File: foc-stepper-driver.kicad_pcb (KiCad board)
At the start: 4 copper layers, 42 x 42 mm, 70 parts, among them CN1 XT30UPB-F30.G.Y, J1 Conn_01x04_Pin, J2 TC2030, J3 CAN_CONNECTOR, J4 USART CONNECTOR, U1 DRV8962DDWR, U2 TYPE-C 16PLT-H10.0, U3 STM32G431CBT6, U6 AS5047P-ATSM, U7 TPS560430XDBVR, U8 SPX3819M5-L-3-3/TR, U9 TCAN3403DRQ1, X1 NX3215SA 32.768KHZ EXS00A-MU0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, X2 NDK NX2016SA-24MHZ-EXS00A-CS1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

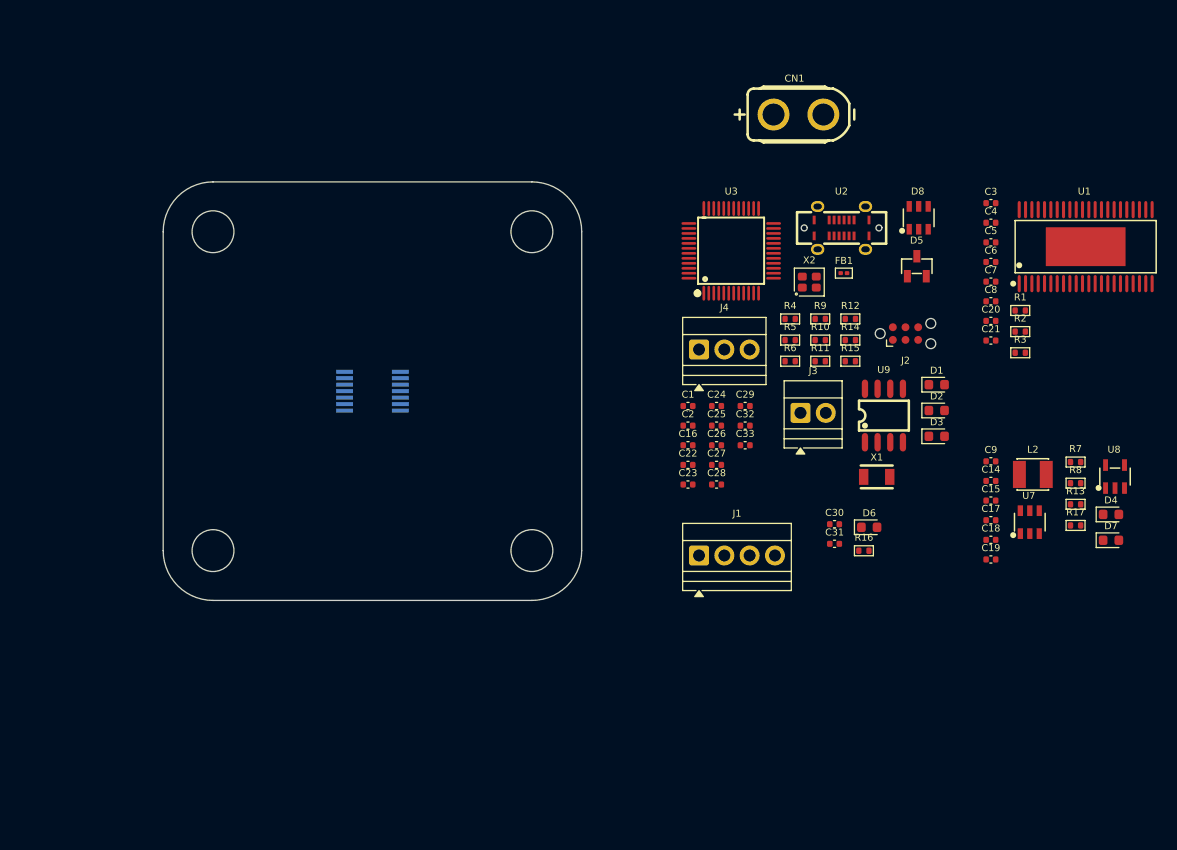
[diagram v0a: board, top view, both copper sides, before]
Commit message: pcb layout
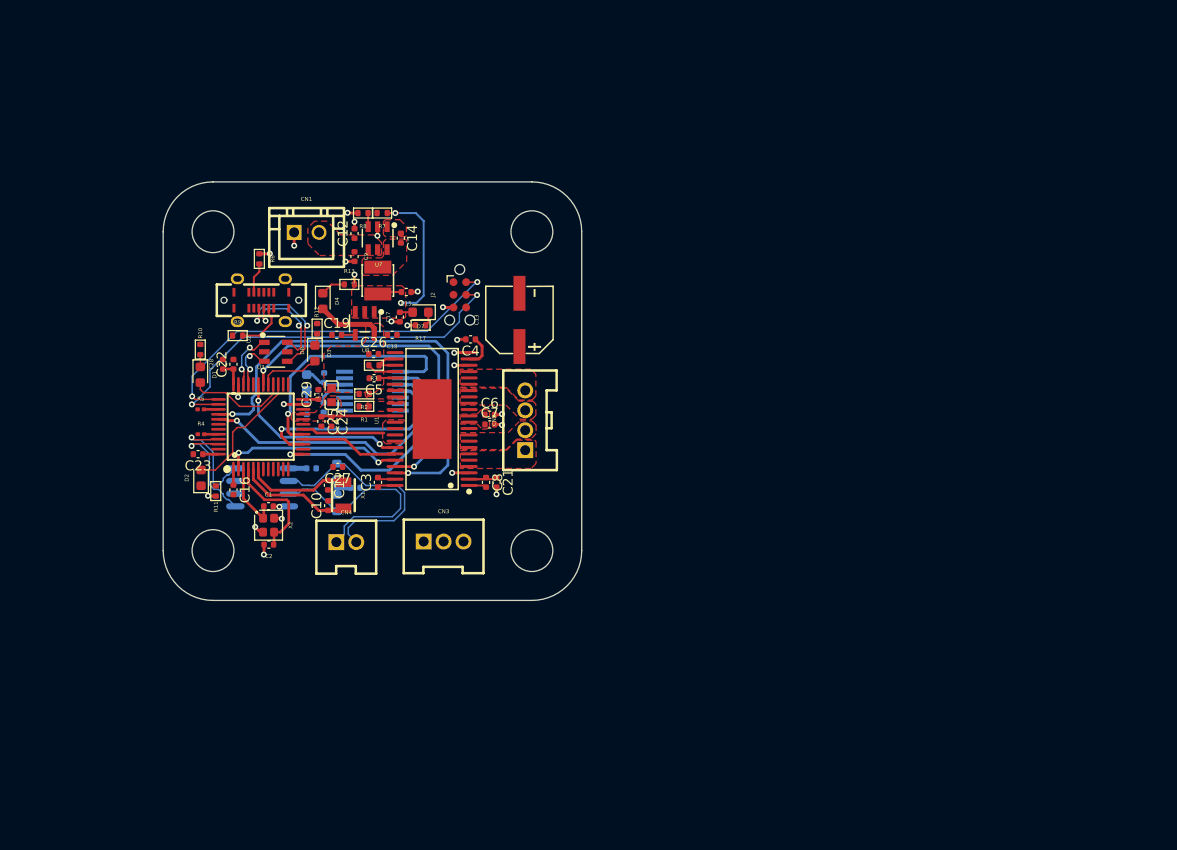
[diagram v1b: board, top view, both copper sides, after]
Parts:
- removed C20: 47u, Capacitor_SMD:C_0402_1005Metric
- removed D5: ESD2CANFD24DBZR, EasyEDA_Lib:SOT-23-3_L2.9-W1.3-P1.90-LS2.4-BL-2
- removed FB1: 120R, PCM_Ferrite_SMD_AKL:Ferrite_0201_0603Metric
- removed J1: Conn_01x04_Pin, TerminalBlock:TerminalBlock_Xinya_XY308-2.54-4P_1x04_P2.54mm_Horizontal
- removed J3: CAN_CONNECTOR, TerminalBlock:TerminalBlock_Xinya_XY308-2.54-2P_1x02_P2.54mm_Horizontal
- removed J4: USART CONNECTOR, TerminalBlock:TerminalBlock_Xinya_XY308-2.54-3P_1x03_P2.54mm_Horizontal
- added C10: 5.1p, Capacitor_SMD:C_0402_1005Metric, F.Cu at (130.9, 96.0)
- added C11: 5.1p, Capacitor_SMD:C_0402_1005Metric, F.Cu at (130.8, 93.9)
- added C12: 100n, Capacitor_SMD:C_0402_1005Metric, F.Cu at (133.5, 68.7)
- added C13: 47uF, EasyEDA_Lib:CAP-SMD_BD6.3-L6.6-W6.6-LS7.3-FD, F.Cu at (150.1, 77.3)
- added CN2: C2839706, EasyEDA_Lib:CONN-TH_PA-4A, F.Cu at (150.6, 87.4)
- added CN3: C2839705, EasyEDA_Lib:CONN-TH_PA-3A, F.Cu at (142.4, 99.6)
- added CN4: C2839704, EasyEDA_Lib:CONN-TH_PA-2A, F.Cu at (132.7, 99.7)
- added L1: BLM18PG121SN1D, EasyEDA_Lib:L0603, F.Cu at (131.2, 84.9)
- C14: value 0.1u -> 100n
- C30, C31, C32, D6, U9: moved to B.Cu
- C33: value 47u -> 4.7n; moved to B.Cu
- C9: value 2.2u -> 10u
- CN1: value XT30UPB-F30.G.Y -> C42391660; footprint EasyEDA_Lib:CONN-TH_XT30UPB-F -> EasyEDA_Lib:CONN-TH_2P-P2.50_HX-2.54MM-2P-ZZ-MS
- R14, R15: footprint PCM_Resistor_SMD_AKL:R_0402_1005Metric -> PCM_Resistor_SMD_AKL:R_0603_1608Metric; moved to B.Cu
- R16: value 100 -> 1k; moved to B.Cu
- R4, R5: footprint PCM_Resistor_SMD_AKL:R_0402_1005Metric -> Capacitor_SMD:C_0201_0603Metric
- moved D4 81.9 mm to (130.3, 75.5), turned to -90 degrees
- moved U8 76.8 mm to (134.5, 77.7), turned to 180 degrees
- moved R8 76.5 mm to (134.3, 66.6), turned to 180 degrees
- moved R13 76.1 mm to (133.0, 73.8)
- moved D2 74.1 mm to (118.1, 93.2), turned to 90 degrees
- moved R7 73.9 mm to (136.3, 66.6), turned to 180 degrees
- moved D1 73.9 mm to (118.0, 82.8), turned to -90 degrees
- moved D7 73.0 mm to (140.1, 76.6), turned to 180 degrees
- moved U7 71.4 mm to (135.8, 69.1), turned to 180 degrees
- moved C19 69.4 mm to (131.7, 78.8)
- moved R17 68.7 mm to (140.1, 77.9), turned to 180 degrees
- moved L2 68.6 mm to (135.8, 73.4), turned to 90 degrees
- moved U1 67.8 mm to (141.3, 87.3), turned to 90 degrees
- moved C3 67.6 mm to (135.8, 93.7), turned to 90 degrees
- moved C9 67.1 mm to (133.5, 71.0), turned to -90 degrees
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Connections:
- net /STM32G431CBT6/STM32_CANFD_RX renamed /STM32G431CBT6/STM32_CANFD+
- net /STM32G431CBT6/STM32_CANFD_TX renamed /STM32G431CBT6/STM32_CANFD-
- net Net-(J3-Pin_1) renamed /STM32G431CBT6/CAN_CONN+
- net Net-(J3-Pin_2) renamed /STM32G431CBT6/CAN_CONN-
- net Net-(U2-DN1) renamed /STM32G431CBT6/USBC_CONN_D-
- net Net-(U2-DP1) renamed /STM32G431CBT6/USBC_CONN_D+
- C19 pad 2: GND -> Net-(U8-BYP)
- C31 pad 2: Net-(D6-K) -> Net-(D6-A)
- C32 pad 1: Net-(U9-VCC) -> +3.3V
- CN1 pad 1: +24V -> GND
- CN1 pad 2: GND -> +24V
- J2 pad 3: /STM32G431CBT6/STM32_NRST -> unconnected-(J2-Pad3)
- R16 pad 1: Net-(D6-A) -> Net-(D6-K)
- U3 pad 14: /DRV8962DDWR/DRV8962_IPROPI1 -> /DRV8962DDWR/DRV8962_IPROPI3
- U3 pad 16: /DRV8962DDWR/DRV8962_IN4 -> /DRV8962DDWR/DRV8962_IN3
- U3 pad 31: /DRV8962DDWR/DRV8962_IN3 -> /DRV8962DDWR/DRV8962_IN4
- U3 pad 8: /DRV8962DDWR/DRV8962_IPROPI3 -> /DRV8962DDWR/DRV8962_IPROPI1
- U6 pad 12: Net-(D6-K) -> Net-(D6-A)
- U8 pad 4: GND -> Net-(U8-BYP)
- U9 pad 3: Net-(U9-VCC) -> +3.3V
- U9 pad 5: +24V -> +3.3V
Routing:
- net /DRV8962DDWR/DRV8962_nSLEEP: track 0.00 -> 46.0 mm, vias 0 -> 2
- net /STM32G431CBT6/STM32_SWCLK: track 0.00 -> 38.5 mm, vias 0 -> 2
- net /STM32G431CBT6/STM32_SWDIO: track 0.00 -> 38.5 mm, vias 0 -> 2
- net /DRV8962DDWR/DRV8962_IN1: track 0.00 -> 34.5 mm, vias 0 -> 2
- net /AS5047P/AS5047P_SPI_MISO: track 0.00 -> 28.9 mm, vias 0 -> 1
- net GND: track 0.00 -> 25.7 mm, vias 0 -> 25
- net /AS5047P/AS5047P_SPI_CSn: track 0.00 -> 25.7 mm, vias 0 -> 1
- net /AS5047P/AS5047P_SPI_CLK: track 0.00 -> 25.4 mm, vias 0 -> 1
- net /STM32G431CBT6/CAN_CONN-: track 0.00 -> 23.8 mm
- net /STM32G431CBT6/CAN_CONN+: track 0.00 -> 23.2 mm
- net /AS5047P/AS5047P_SPI_MOSI: track 0.00 -> 21.8 mm, vias 0 -> 1
- net +5V: track 0.00 -> 21.3 mm, vias 0 -> 2
- net /DRV8962DDWR/DRV8962_IN2: track 0.00 -> 18.2 mm, vias 0 -> 2
- net /DRV8962DDWR/DRV8962_IN4: track 0.00 -> 18.2 mm, vias 0 -> 2
- net +3.3V: track 0.00 -> 15.7 mm
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- added copper zone on F.Cu, net +24V
- added copper zone on F.Cu, net +3.3V
- added copper zone on F.Cu, net +3.3VA
- added copper zone on F.Cu, net +5V
- added copper zone on F.Cu, net /DRV8962DDWR/DRV8962_EN
- added copper zone on F.Cu, net /DRV8962DDWR/DRV8962_IPROPI1
- added copper zone on F.Cu, net /DRV8962DDWR/DRV8962_IPROPI3
- added copper zone on F.Cu, net /DRV8962DDWR/DRV8962_OUT1
- added copper zone on F.Cu, net /DRV8962DDWR/DRV8962_OUT2
- added copper zone on F.Cu, net /DRV8962DDWR/DRV8962_OUT3
- added copper zone on F.Cu, net /DRV8962DDWR/DRV8962_OUT4
- added copper zone on F.Cu, net Net-(U7-CB)
- added copper zone on F.Cu, net Net-(U7-SW)
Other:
- board text added: "${REFERENCE}"

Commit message: update
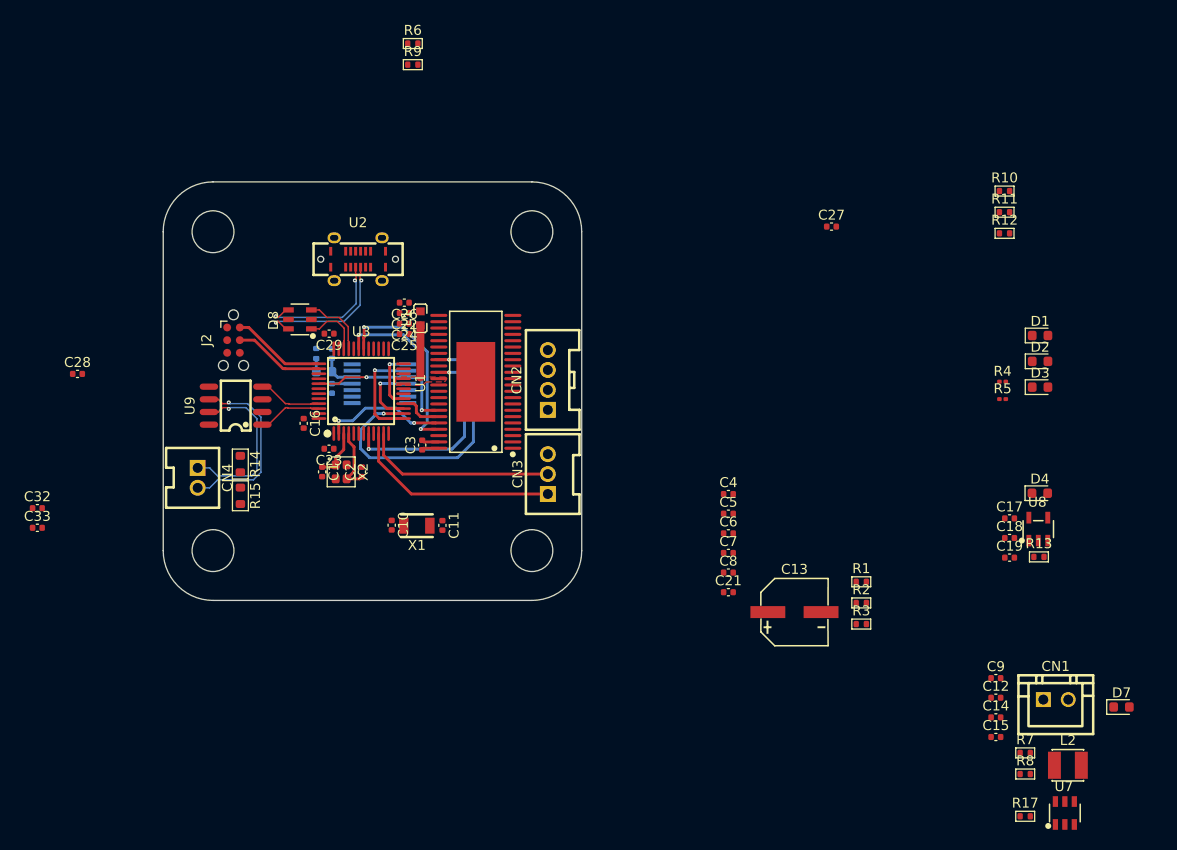
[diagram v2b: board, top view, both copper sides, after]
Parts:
- C32, C33, R14, R15, U9: moved to F.Cu
- moved U7 89.9 mm to (204.8, 126.8), turned to 0 degrees
- moved CN1 88.6 mm to (203.9, 115.5)
- moved R8 87.1 mm to (200.8, 122.9), turned to 0 degrees
- moved D2 85.0 mm to (202.3, 81.5), turned to 0 degrees
- moved L2 84.6 mm to (205.1, 122.0), turned to 0 degrees
- moved D1 84.4 mm to (202.3, 78.9), turned to 0 degrees
- moved R7 84.3 mm to (200.8, 120.8), turned to 0 degrees
- moved R11 84.0 mm to (198.7, 66.5), turned to 0 degrees
- moved R10 82.3 mm to (198.7, 64.4), turned to 0 degrees
- moved D7 80.7 mm to (210.5, 116.2), turned to 0 degrees
- moved R4 80.6 mm to (198.5, 83.5)
- moved R5 80.5 mm to (198.5, 85.3)
- moved C12 79.5 mm to (197.9, 115.3), turned to 0 degrees
- moved R17 78.2 mm to (200.8, 127.2), turned to 0 degrees
- moved C9 77.0 mm to (197.9, 113.3), turned to 0 degrees
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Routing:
- net /DRV8962DDWR/DRV8962_nSLEEP: track 46.0 -> 0.00 mm, vias 2 -> 0
- net /DRV8962DDWR/DRV8962_IPROPI3: track 0.00 -> 30.4 mm, vias 0 -> 2
- net /STM32G431CBT6/STM32_SWCLK: track 38.5 -> 9.12 mm, vias 2 -> 0
- net /STM32G431CBT6/STM32_SWDIO: track 38.5 -> 9.44 mm, vias 2 -> 0
- net GND: track 25.7 -> 0.00 mm, vias 25 -> 0
- net /STM32G431CBT6/STM32_USART_TX: track 0.00 -> 21.1 mm
- net /DRV8962DDWR/DRV8962_IPROPI1: track 0.00 -> 20.7 mm, vias 0 -> 2
- net /AS5047P/AS5047P_SPI_MISO: track 28.9 -> 9.19 mm
- net /STM32G431CBT6/STM32_USART_RX: track 0.00 -> 19.4 mm
- net +5V: track 21.3 -> 2.08 mm, vias 2 -> 0
- net /AS5047P/AS5047P_SPI_CSn: track 25.7 -> 6.47 mm
- net +3.3V: track 15.7 -> 0.00 mm
- net /DRV8962DDWR/DRV8962_IN1: track 34.5 -> 19.1 mm
- net /AS5047P/AS5047P_SPI_CLK: track 25.4 -> 10.8 mm
- net /AS5047P/AS5047P_SPI_MOSI: track 21.8 -> 7.24 mm
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- removed copper zone on F.Cu, net +24V
- removed copper zone on F.Cu, net +3.3V
- removed copper zone on F.Cu, net +5V
- removed copper zone on F.Cu, net /DRV8962DDWR/DRV8962_EN
- removed copper zone on F.Cu, net /DRV8962DDWR/DRV8962_IPROPI1
- removed copper zone on F.Cu, net /DRV8962DDWR/DRV8962_IPROPI3
- removed copper zone on F.Cu, net /DRV8962DDWR/DRV8962_OUT1
- removed copper zone on F.Cu, net /DRV8962DDWR/DRV8962_OUT2
- removed copper zone on F.Cu, net /DRV8962DDWR/DRV8962_OUT3
- removed copper zone on F.Cu, net /DRV8962DDWR/DRV8962_OUT4
- removed copper zone on F.Cu, net Net-(U7-CB)
- removed copper zone on F.Cu, net Net-(U7-SW)

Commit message: update route
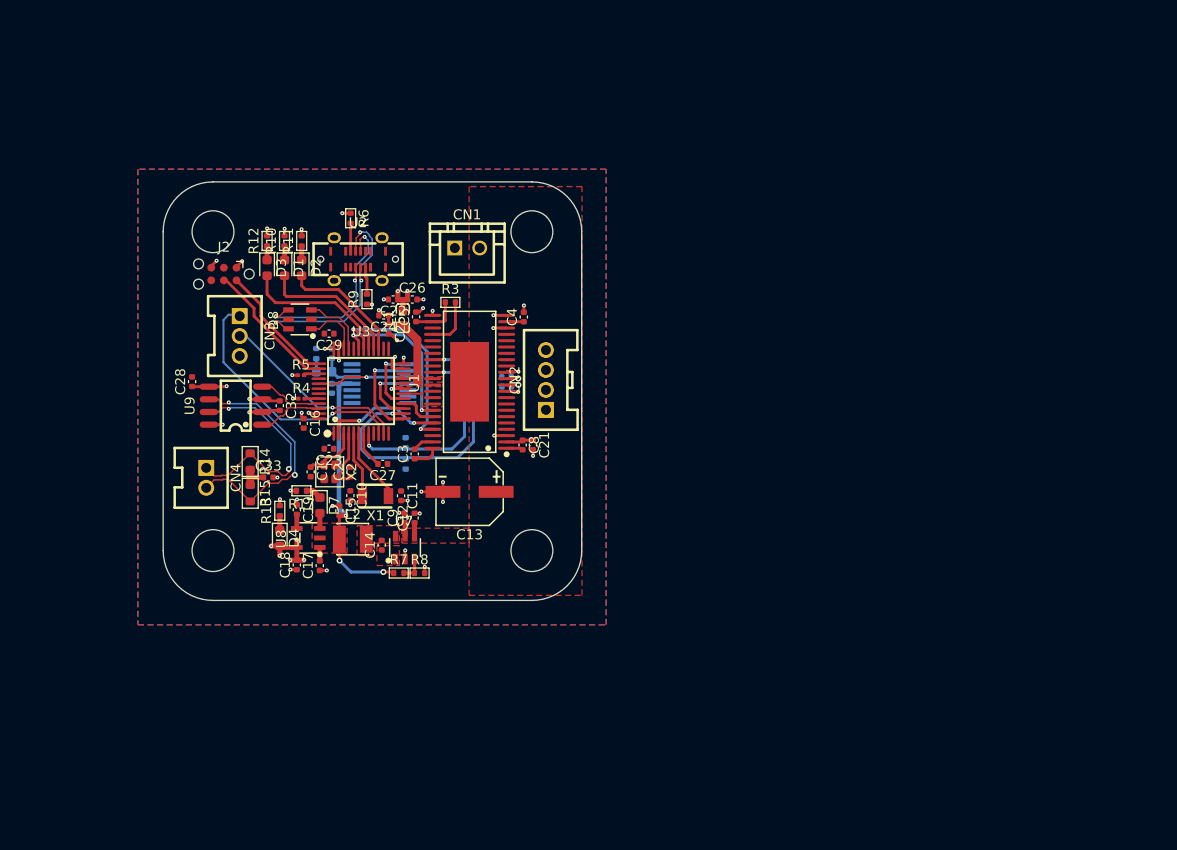
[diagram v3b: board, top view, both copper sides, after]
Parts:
- C6, C7, R1, R2: moved to B.Cu
- moved D7 83.0 mm to (130.0, 96.0), turned to -90 degrees
- moved R17 79.6 mm to (128.2, 94.5), turned to 180 degrees
- moved D3 78.5 mm to (124.7, 72.1), turned to -90 degrees
- moved D4 76.4 mm to (126.0, 99.2), turned to -90 degrees
- moved R13 76.3 mm to (126.0, 96.5), turned to 90 degrees
- moved D1 76.1 mm to (126.5, 72.1), turned to -90 degrees
- moved L2 75.3 mm to (133.3, 99.3)
- moved D2 74.7 mm to (128.2, 72.1), turned to -90 degrees
- moved CN1 74.4 mm to (144.8, 70.1)
- moved R12 74.0 mm to (124.7, 69.4), turned to 90 degrees
- moved U8 73.3 mm to (128.9, 99.2), turned to 90 degrees
- moved R10 72.4 mm to (126.5, 69.4), turned to 90 degrees
- moved C19 71.7 mm to (127.7, 96.4), turned to -90 degrees
- moved C18 71.6 mm to (127.7, 101.9), turned to 90 degrees
- moved U7 71.4 mm to (138.6, 100.2)
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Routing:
- net GND: track 0.00 -> 38.7 mm, vias 0 -> 41
- net +5V: track 2.08 -> 34.2 mm, vias 0 -> 3
- net +3.3V: track 0.00 -> 22.2 mm, vias 0 -> 16
- net /STM32G431CBT6/STM32_DEBUG_3: track 0.00 -> 15.1 mm
- net /STM32G431CBT6/STM32_DEBUG_2: track 0.00 -> 13.9 mm
- net /STM32G431CBT6/STM32_DEBUG_1: track 0.00 -> 12.5 mm
- net +24V: track 0.00 -> 11.1 mm, vias 0 -> 2
- net /STM32G431CBT6/USBC_CONN_D+: track 14.7 -> 23.1 mm, vias 2 -> 3
- net /STM32G431CBT6/OSC_OUT: track 0.00 -> 7.52 mm
- net /STM32G431CBT6/USBC_CONN_D-: track 14.1 -> 20.9 mm, vias 2 -> 3
- net /STM32G431CBT6/OSC_IN: track 0.00 -> 6.64 mm
- net /STM32G431CBT6/CAN_CONN-: track 18.6 -> 25.1 mm, vias 1 -> 2
- net /STM32G431CBT6/CAN_CONN+: track 17.3 -> 23.6 mm, vias 1 -> 2
- net /DRV8962DDWR/DRV8962_nFAULT: track 0.00 -> 5.18 mm
- net /DRV8962DDWR/DRV8962_DVDD: track 0.00 -> 4.80 mm
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- added copper zone on F.Cu, net +24V
- added copper zone on In2.Cu, net +3.3V
- added copper zone on F.Cu, net +5V
- added copper zone on F.Cu, net /DRV8962DDWR/DRV8962_EN
- added copper zone on B.Cu, net GND
- added copper zone on F.Cu, net GND
- added copper zone on In1.Cu, net GND
- added copper zone on F.Cu, net Net-(U7-CB)
- added copper zone on F.Cu, net Net-(U7-SW)
